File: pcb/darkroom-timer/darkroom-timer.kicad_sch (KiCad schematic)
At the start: 15 parts, among them J3 Conn_01x02_Socket, K1 Relay_DPDT, SW1 RotaryEncoder_Switch_MP, SW4 Start Switch, U3 PC817

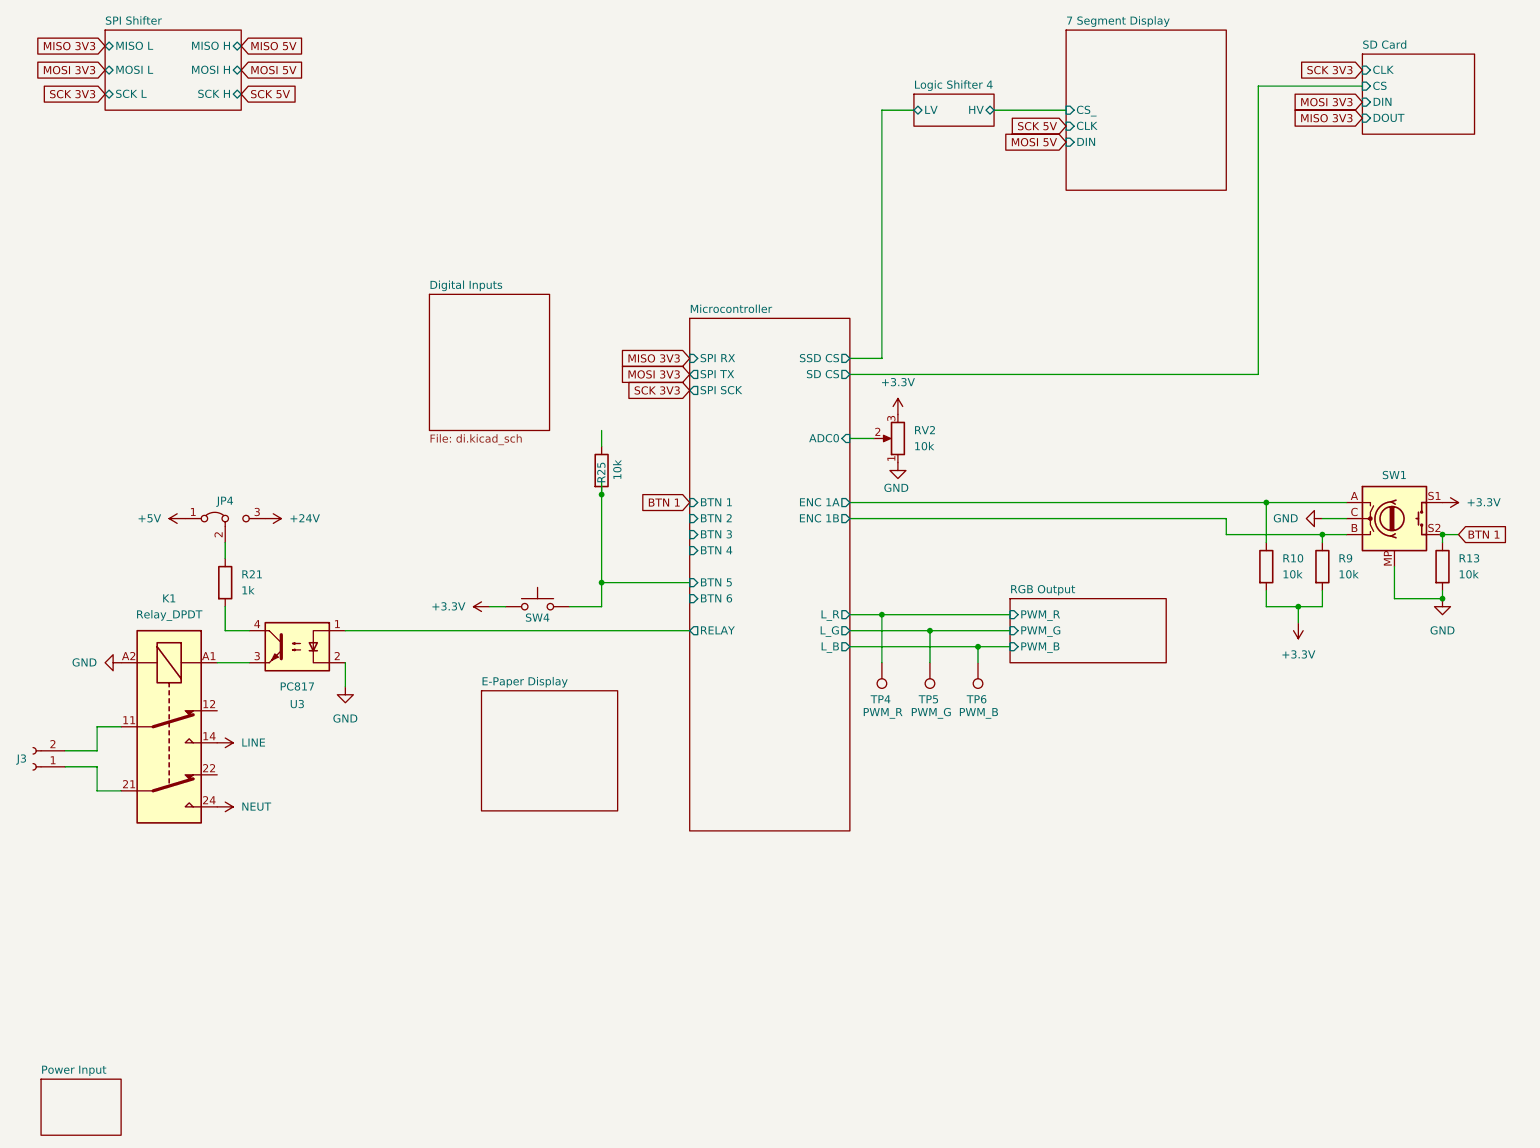
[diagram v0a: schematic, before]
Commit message: PCB Ready
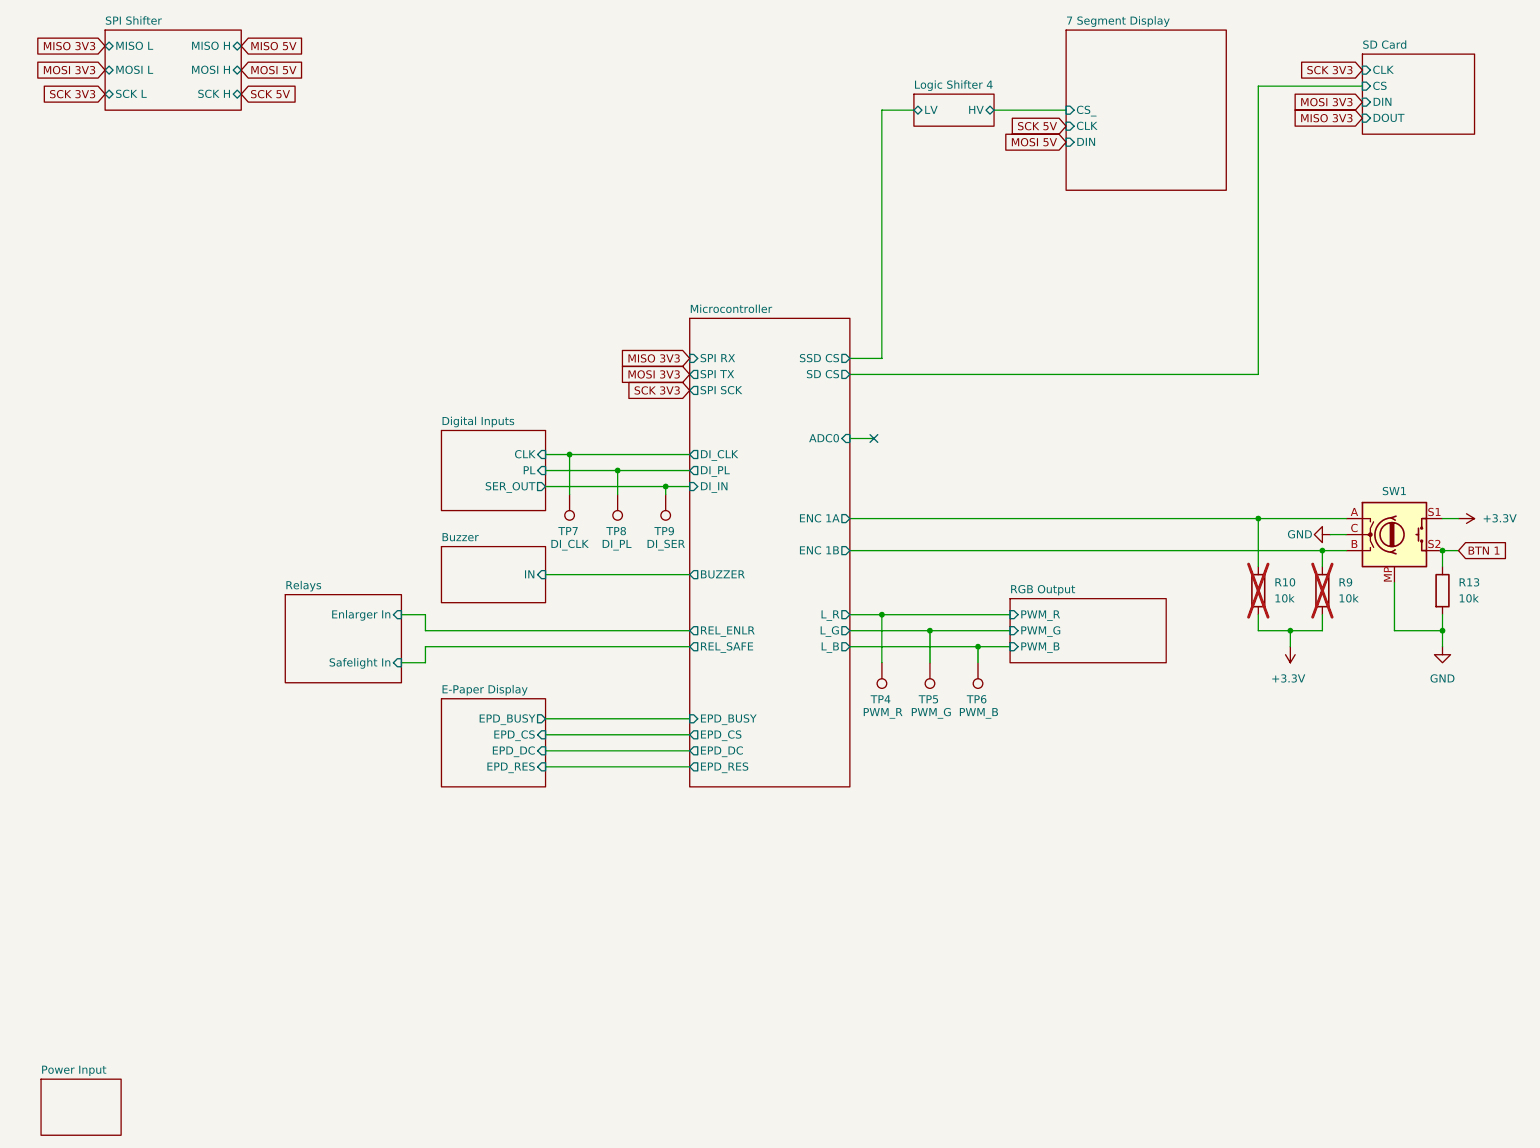
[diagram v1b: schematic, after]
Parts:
- removed J3: Conn_01x02_Socket, Connector_Wire:SolderWire-1.5sqmm_1x02_P7.8mm_D1.7mm_OD3.9mm, symbol Connector:Conn_01x02_Socket
- removed JP4: Jumper_3_Bridged12, PCM_SparkFun-Jumper:Jumper_3_NC-1_Trace, symbol Jumper:Jumper_3_Bridged12
- removed K1: Relay_DPDT, Relay_THT:Relay_DPDT_Panasonic_JW2, symbol Relay:Relay_DPDT
- removed R21: 1k, Resistor_SMD:R_0201_0603Metric, symbol Device:R
- removed R25: 10k, Resistor_SMD:R_0201_0603Metric, symbol Device:R
- removed RV2: 10k, Potentiometer_THT:Potentiometer_Alps_RK09K_Single_Vertical, symbol Device:R_Potentiometer
- removed SW4: Start Switch, symbol Switch:SW_Push
- removed U3: PC817, Package_DIP:DIP-4_W7.62mm, symbol Isolator:PC817
- added TP7: DI_CLK, TestPoint:TestPoint_Pad_D1.5mm, symbol Connector:TestPoint
- added TP8: DI_PL, TestPoint:TestPoint_Pad_D1.5mm, symbol Connector:TestPoint
- added TP9: DI_SER, TestPoint:TestPoint_Pad_D1.5mm, symbol Connector:TestPoint
- R10, R9: footprint Resistor_SMD:R_0201_0603Metric -> Resistor_SMD:R_0805_2012Metric; Placement Optional -> (none); now not fitted
- R13: footprint Resistor_SMD:R_0201_0603Metric -> Resistor_SMD:R_0805_2012Metric; Placement Optional -> (none)
- SW1: footprint Rotary_Encoder:RotaryEncoder_Alps_EC11E-Switch_Vertical_H20mm_MountingHoles -> Frank:RotaryEncoder_Alps_EC11E-Switch_Vertical_3D; InvenTree Part # (none) -> 640; Placement Required -> (none)
- TP4, TP5, TP6: Placement Required -> (none)
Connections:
- new net Digital Inputs/CLK: TP7.1
- new net Digital Inputs/PL: TP8.1
- new net Digital Inputs/SER_OUT: TP9.1
- no-connect marks 0 -> 1
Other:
- added sheet Buzzer (buzzer.kicad_sch)
- added sheet Relays (relays.kicad_sch)
- sheet Digital Inputs ports: added CLK, PL, SER_OUT; removed none
- sheet E-Paper Display ports: added EPD_BUSY, EPD_CS, EPD_DC, EPD_RES; removed none
- sheet Microcontroller ports: added BUZZER, DI_CLK, DI_IN, DI_PL, EPD_BUSY, EPD_CS, EPD_DC, EPD_RES, REL_ENLR, REL_SAFE; removed BTN 1, BTN 2, BTN 3, BTN 4, BTN 5, BTN 6, RELAY
- moved on the sheet: R13, SW1
